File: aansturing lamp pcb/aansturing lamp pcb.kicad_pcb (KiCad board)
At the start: 2 copper layers, 35 x 23 mm, 16 parts, among them J4 Conn_01x06_Pin, U1 LM317_SOT-223

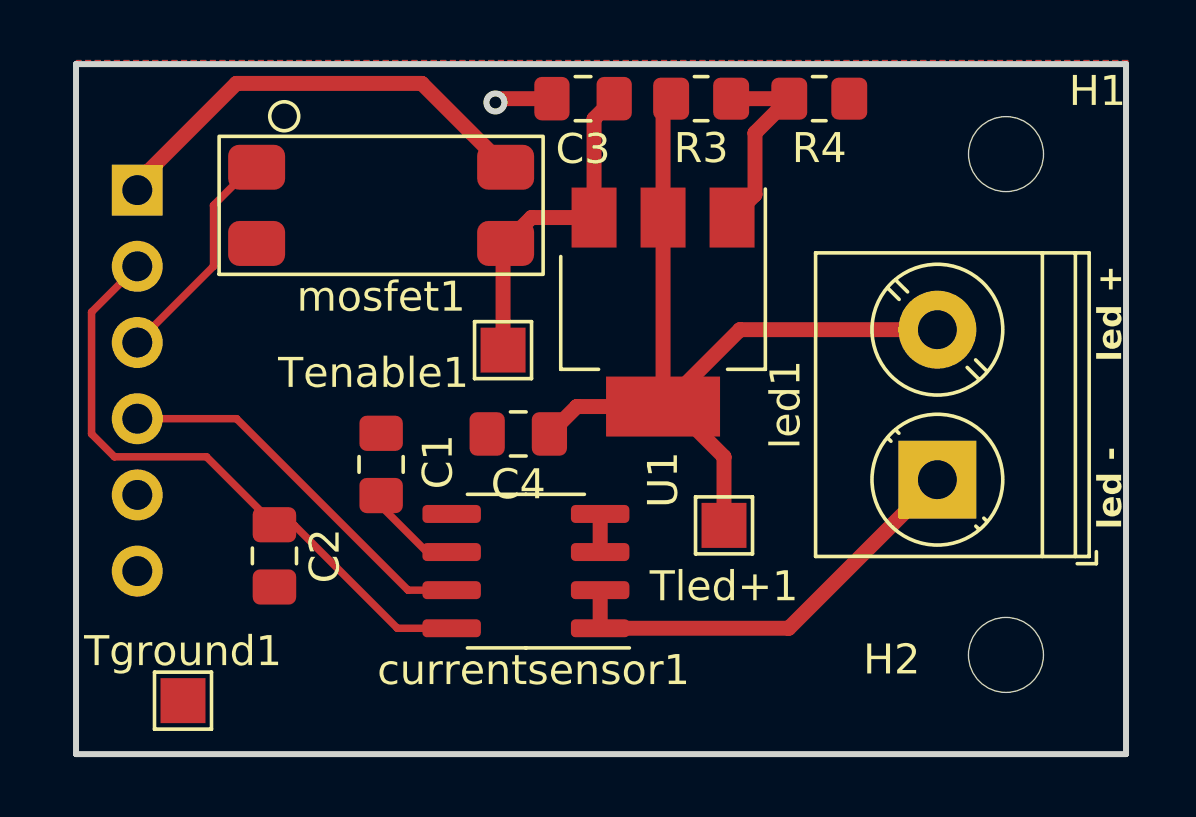
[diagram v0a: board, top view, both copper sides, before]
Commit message: ok
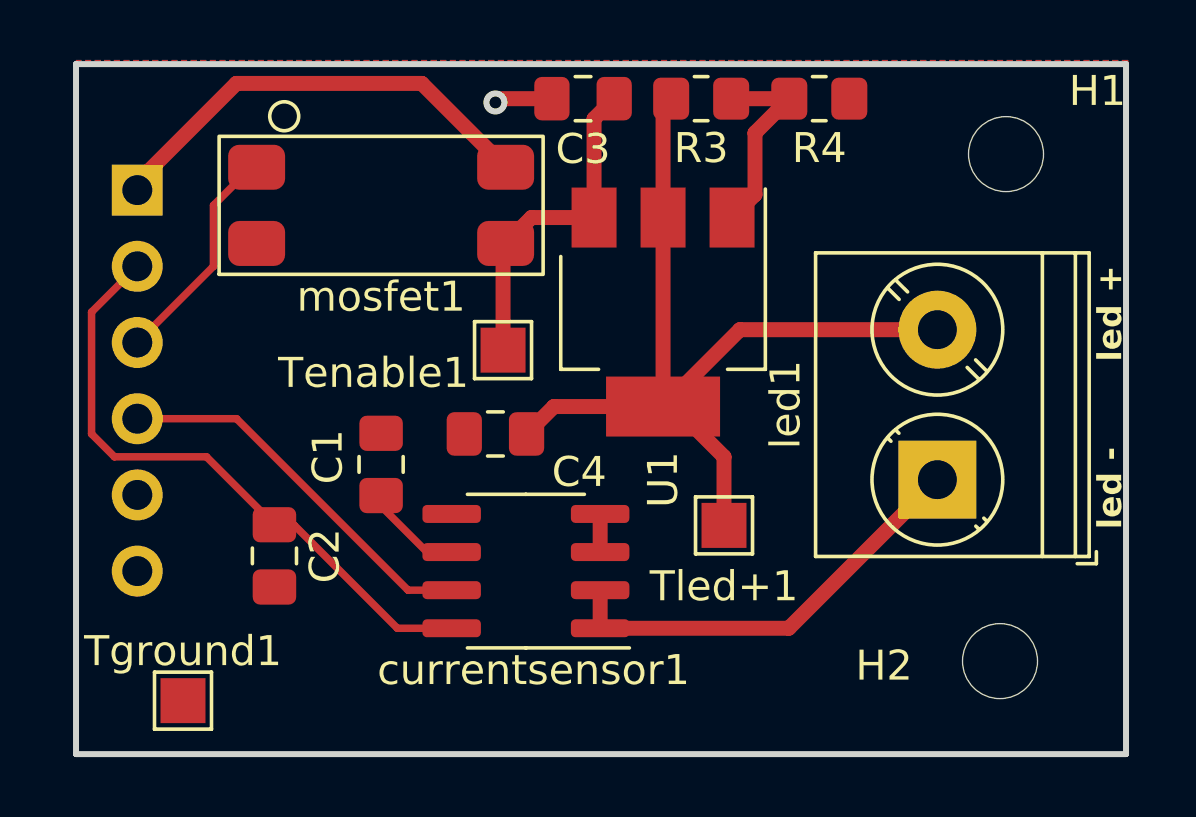
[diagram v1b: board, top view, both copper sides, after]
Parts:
- moved C4 0.76 mm to (94.0, 84.3)
- moved H2 0.23 mm to (110.9, 91.9)
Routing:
- net /led+: track 29.8 -> 30.5 mm
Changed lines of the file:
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@@
   )
   (footprint "MountingHole:MountingHole_2.5mm" (layer "F.Cu")
-    (at 110.998 91.694)
+    (at 110.9 91.9)
     (descr "Mounting Hole 2.5mm, no annular")
     (tags "mounting hole 2.5mm no annular")
@@
     (property "ki_keywords" "mounting hole")
     (attr exclude_from_pos_files)
-    (fp_text reference "H2" (at -3.808 0.154) (layer "F.SilkS")
+    (fp_text reference "H2" (at -3.966 0.154) (layer "F.SilkS")
         (effects (font (size 1 1) (thickness 0.15)))
     )
@@
     (fp_circle (center 0 0) (end 2.75 0)
       (stroke (width 0.05) (type solid)) (fill none) (layer "F.CrtYd"))
-    (pad "" np_thru_hole circle (at 0 0) (size 2.5 2.5) (drill 2.5) (layers "*.Cu" "*.Mask"))
+    (pad "" np_thru_hole circle (at -0.1 0) (size 2.5 2.5) (drill 2.5) (layers "F&B.Cu" "*.Mask"))
   )
   (footprint "Capacitor_SMD:C_0805_2012Metric_Pad1.18x1.45mm_HandSolder" (layer "F.Cu")
-    (at 94.742 84.328 180)
+    (at 93.98 84.328 180)
     (descr "Capacitor SMD 0805 (2012 Metric), square (rectangular) end terminal, IPC_7351 nominal with elongated pad for handsoldering. (Body size source: IPC-SM-782 page 76, https://www.pcb-3d.com/wordpress/wp-content/uploads/ipc-sm-782a_amendment_1_and_2.pdf, https://docs.google.com/spreadsheets/d/1BsfQQcO9C6DZCsRaXUlFlo91Tg2WpOkGARC1WS5S8t0/edit?usp=sharing), generated with kicad-footprint-generator")
     (tags "capacitor handsolder")
@@
     (property "ki_keywords" "capacitor cap")
     (attr smd)
-    (fp_text reference "C4" (at 0 -1.68) (layer "F.SilkS")
+    (fp_text reference "C4" (at -2.794 -1.27) (layer "F.SilkS")
         (effects (font (size 1 1) (thickness 0.15)))
     )
@@
     (property "ki_keywords" "capacitor cap")
     (attr smd)
-    (fp_text reference "C1" (at 0.0872 1.8924 90) (layer "F.SilkS")
+    (fp_text reference "C1" (at 0.254 -1.778 90) (layer "F.SilkS")
         (effects (font (size 1 1) (thickness 0.15)))
     )
@@
   (segment (start 94.319996 77.978) (end 94.234 78.063996) (width 0.5) (layer "F.Cu") (net 8))
   (segment (start 97.268 73.8225) (end 97.9385 73.152) (width 0.5) (layer "F.Cu") (net 8))
+  (segment (start 95.9315 83.414) (end 95.0175 84.328) (width 0.5) (layer "F.Cu") (net 9))
+  (segment (start 99.568 83.414) (end 95.9315 83.414) (width 0.5) (layer "F.Cu") (net 9))
   (segment (start 101.6 85.09) (end 101.6 87.376) (width 0.5) (layer "F.Cu") (net 9))
   (segment (start 99.568 73.422) (end 99.838 73.152) (width 0.5) (layer "F.Cu") (net 9))
   (segment (start 99.568 83.414) (end 99.924 83.414) (width 0.5) (layer "F.Cu") (net 9))
-  (segment (start 96.6935 83.414) (end 95.7795 84.328) (width 0.5) (layer "F.Cu") (net 9))
   (segment (start 99.568 77.114) (end 99.568 73.422) (width 0.5) (layer "F.Cu") (net 9))
   (segment (start 99.568 77.114) (end 99.568 83.414) (width 0.5) (layer "F.Cu") (net 9))
-  (segment (start 99.568 83.414) (end 96.6935 83.414) (width 0.5) (layer "F.Cu") (net 9))
   (segment (start 102.13 80.852) (end 99.568 83.414) (width 0.5) (layer "F.Cu") (net 9))
   (segment (start 99.924 83.414) (end 101.6 85.09) (width 0.5) (layer "F.Cu") (net 9))
